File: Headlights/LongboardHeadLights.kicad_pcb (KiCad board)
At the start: 2 copper layers, 76.2 x 10.8 mm, 16 parts, among them P1 CONN_01X03, U1 AL8805

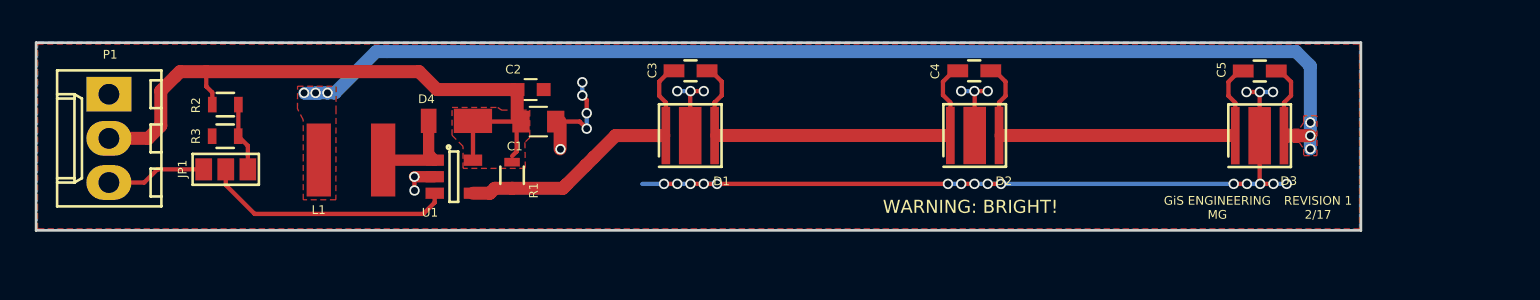
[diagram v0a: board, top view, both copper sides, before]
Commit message: updating designs for newest revision; removing unneeded files
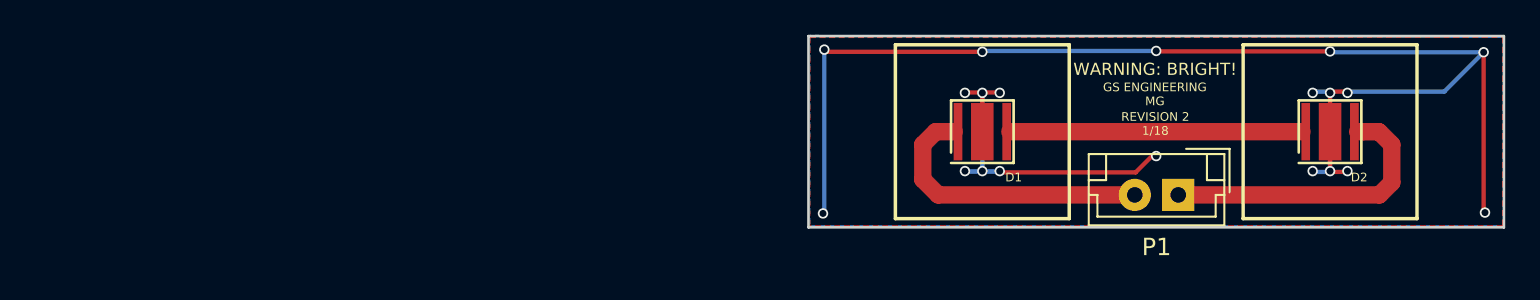
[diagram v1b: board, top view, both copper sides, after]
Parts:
- removed C1: 4.7uF, Capacitors_SMD:C_0805
- removed C2: 2.2uF, Capacitors_SMD:C_0603
- removed C3, C4, C5: 1uF, Capacitors_SMD:C_0603_HandSoldering
- removed D3: LED, LEDs:LED-XP-G_CREE
- removed D4: D_Schottky, Light_Parts:PowerDI-123
- removed JP1: JUMPER3, Connect:GS3
- removed L1: INDUCTOR, Light_Parts:Inductor5x5
- removed R1: 0.3, Resistors_SMD:R_0603
- removed R2: 38000, Resistors_SMD:R_0603
- removed R3: 10000, Resistors_SMD:R_0603
- removed U1: AL8805, TO_SOT_Packages_SMD:SOT-23-5
- P1: footprint Connectors_Molex:Molex_KK-6410-03_03x2.54mm_Straight -> Connectors_JST:JST_EH_B02B-EH-A_02x2.50mm_Straight
- moved P1 61.8 mm to (191.9, 94.9), turned to 180 degrees
- moved D2 20.4 mm to (200.6, 91.2)
- moved D1 16.8 mm to (180.6, 91.2)
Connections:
- D1 pad 2: Net-(C3-Pad1) -> Net-(D1-Pad2)
- D2 pad 1: Net-(C4-Pad2) -> Net-(D2-Pad1)
- P1 pad 1: GND -> Net-(D2-Pad1)
- P1 pad 2: VCC -> Net-(D1-Pad2)
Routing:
- net Net-(C5-Pad2): track 69.8 -> 0.00 mm, vias 6 -> 0
- net VCC: track 37.6 -> 0.00 mm
- net GND: track 61.6 -> 93.1 mm, vias 31 -> 20
- net Net-(C4-Pad2): track 22.2 -> 0.00 mm
- net Net-(D2-Pad1): track 0.00 -> 17.1 mm
- net Net-(C3-Pad1): track 17.1 -> 0.00 mm
- net Net-(D1-Pad2): track 0.00 -> 16.6 mm
- net /CTRL: track 14.4 -> 0.00 mm
- net /CTRL_EXT: track 5.77 -> 0.00 mm
- net Net-(D4-Pad2): track 5.65 -> 0.00 mm
- net Net-(D1-Pad1): track 22.0 -> 16.8 mm
- net Net-(JP1-Pad1): track 4.25 -> 0.00 mm
- removed copper zone on F.Cu, net Net-(C5-Pad2)
- removed copper zone on F.Cu, net VCC
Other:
- board size 76.2 x 10.8 mm -> 40 x 11 mm
- net class Default: clearance 0.2 -> 0
- rule trace_clearance: 0.2 -> 0
- board text added: "GS ENGINEERING MG"
- board text added: "REVISION 2 1/18"
- board text removed: "GiS ENGINEERING MG"
- board text removed: "REVISION 1 2/17"
